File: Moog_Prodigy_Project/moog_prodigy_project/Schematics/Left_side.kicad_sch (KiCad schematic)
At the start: 86 parts, among them Q1 CA3046, Q15 BC549, Q2 CA3046, Q4 CA3046, Q6 BC549, U1 LT1011CN8, U11 +12V, U12 +12V, U15 +12V, U16 +12V, U17 +12V, U18 +12V, U19 +12V, U20 +12V, U21 +12V, U2A OPA134, U2B OPA134, U3 +12V, U4 +12V, U41 +12V, U5 NE5532, U55 -12V, U56 -12V, U57 -12V, U58 -12V, U59 -12V, U6 LT1011CN8, U60 -12V, U61 -12V, U62 -12V, U63 -12V, U64 +12V, U65 +12V, U66 -12V, U7 AD8066ARM, U8 NE5532

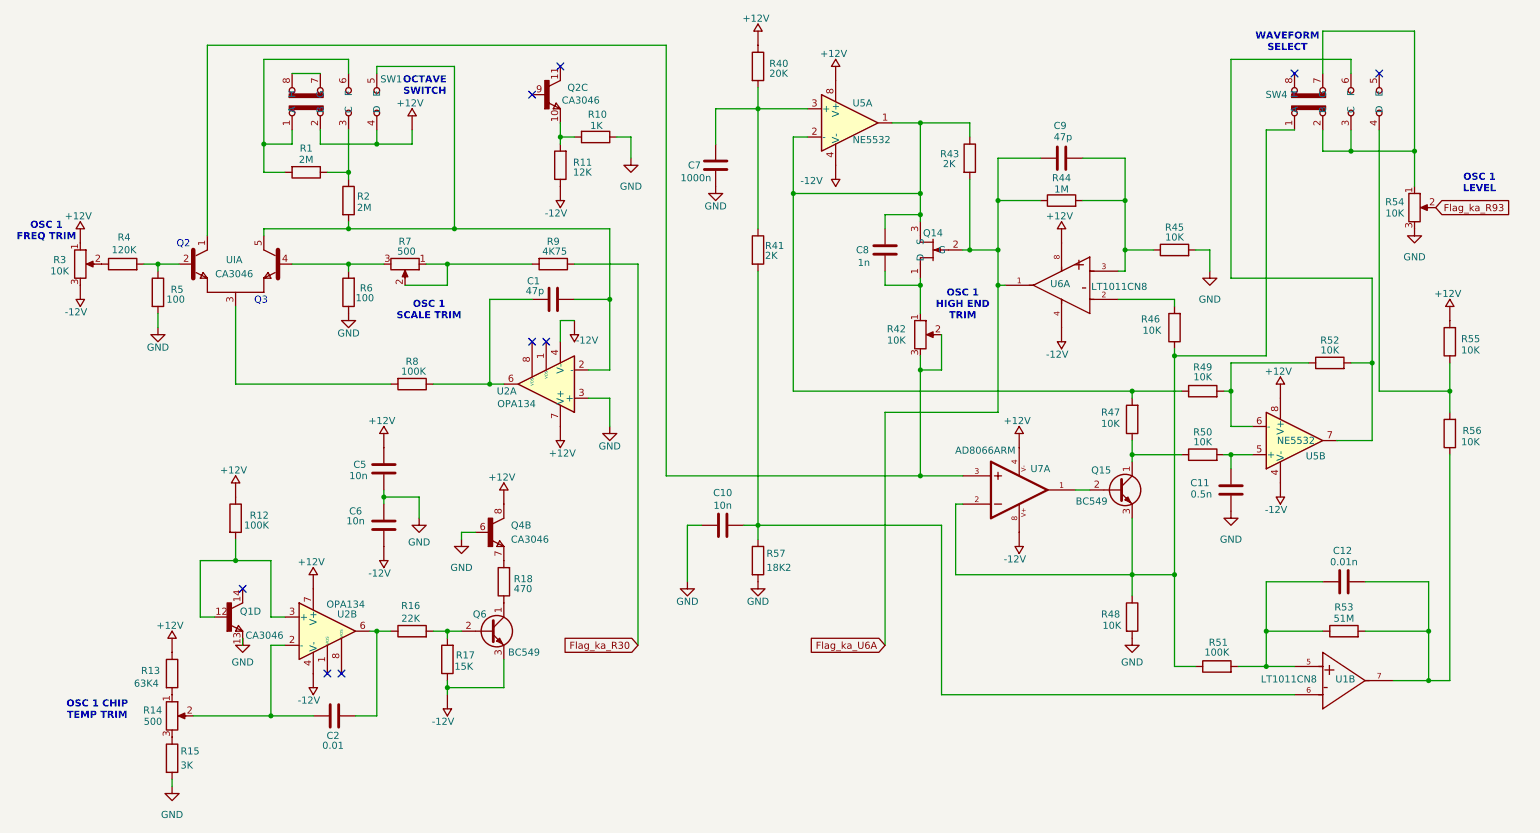
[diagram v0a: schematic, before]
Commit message: New update footprints
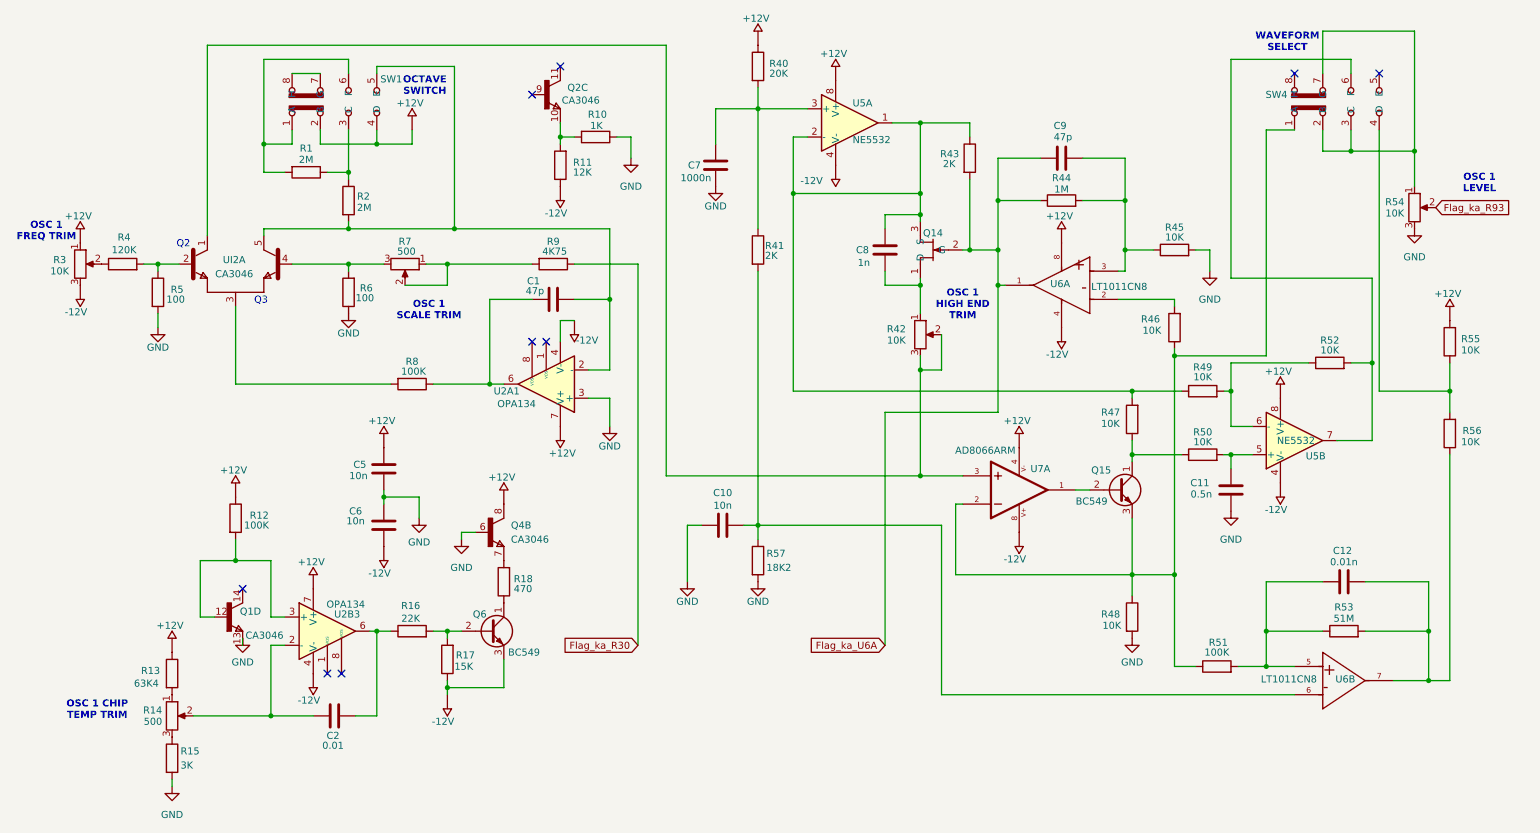
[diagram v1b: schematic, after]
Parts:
- renumbered U2A to U2A1, U2B to U2B3, U1 to U6, UI to UI2
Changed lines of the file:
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@@
 		(on_board yes)
 		(dnp no)
-		(property "Reference" "U2A"
+		(property "Reference" "U2A1"
 			(at 100.838 83.82 0)
 			(effects
@@
 			(project "moog_prodigy_project"
 				(path "/db469bdb-b6c3-4a16-9199-d4e6b8d556e8/2ede1db1-77b0-45c3-aa08-ac2fbfd2e808"
-					(reference "U2A")
+					(reference "U2A1")
 					(unit 1)
 				)
@@
 		(on_board yes)
 		(dnp no)
-		(property "Reference" "U2B"
+		(property "Reference" "U2B3"
 			(at 72.136 123.952 0)
 			(effects
@@
 			(project "moog_prodigy_project"
 				(path "/db469bdb-b6c3-4a16-9199-d4e6b8d556e8/2ede1db1-77b0-45c3-aa08-ac2fbfd2e808"
-					(reference "U2B")
+					(reference "U2B3")
 					(unit 1)
 				)
@@
 		(on_board yes)
 		(dnp no)
-		(property "Reference" "U1"
+		(property "Reference" "U6"
 			(at 251.714 135.636 0)
 			(effects
@@
 			(project ""
 				(path "/db469bdb-b6c3-4a16-9199-d4e6b8d556e8/2ede1db1-77b0-45c3-aa08-ac2fbfd2e808"
-					(reference "U1")
+					(reference "U6")
 					(unit 2)
 				)
@@
 		(on_board yes)
 		(dnp no)
-		(property "Reference" "UI"
+		(property "Reference" "UI2"
 			(at 51.816 60.198 0)
 			(effects
@@
 			(project ""
 				(path "/db469bdb-b6c3-4a16-9199-d4e6b8d556e8/2ede1db1-77b0-45c3-aa08-ac2fbfd2e808"
-					(reference "UI")
+					(reference "UI2")
 					(unit 1)
 				)

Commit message: Footpring fix 2
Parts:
- UI2: footprint (none) -> CA3046:DIL14
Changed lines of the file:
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@@
 			)
 		)
-		(property "Footprint" ""
+		(property "Footprint" "CA3046:DIL14"
 			(at 52.07 60.96 0)
 			(effects
